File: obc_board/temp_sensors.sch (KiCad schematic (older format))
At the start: 84 parts, among them U10 BMM150, U4 LTC4304CMSTRPBF, U5 MCP9600-E_MX, U6 MCP9600-E_MX, U7 MCP9600-E_MX, U8 MCP9600-E_MX, U9 BMI160

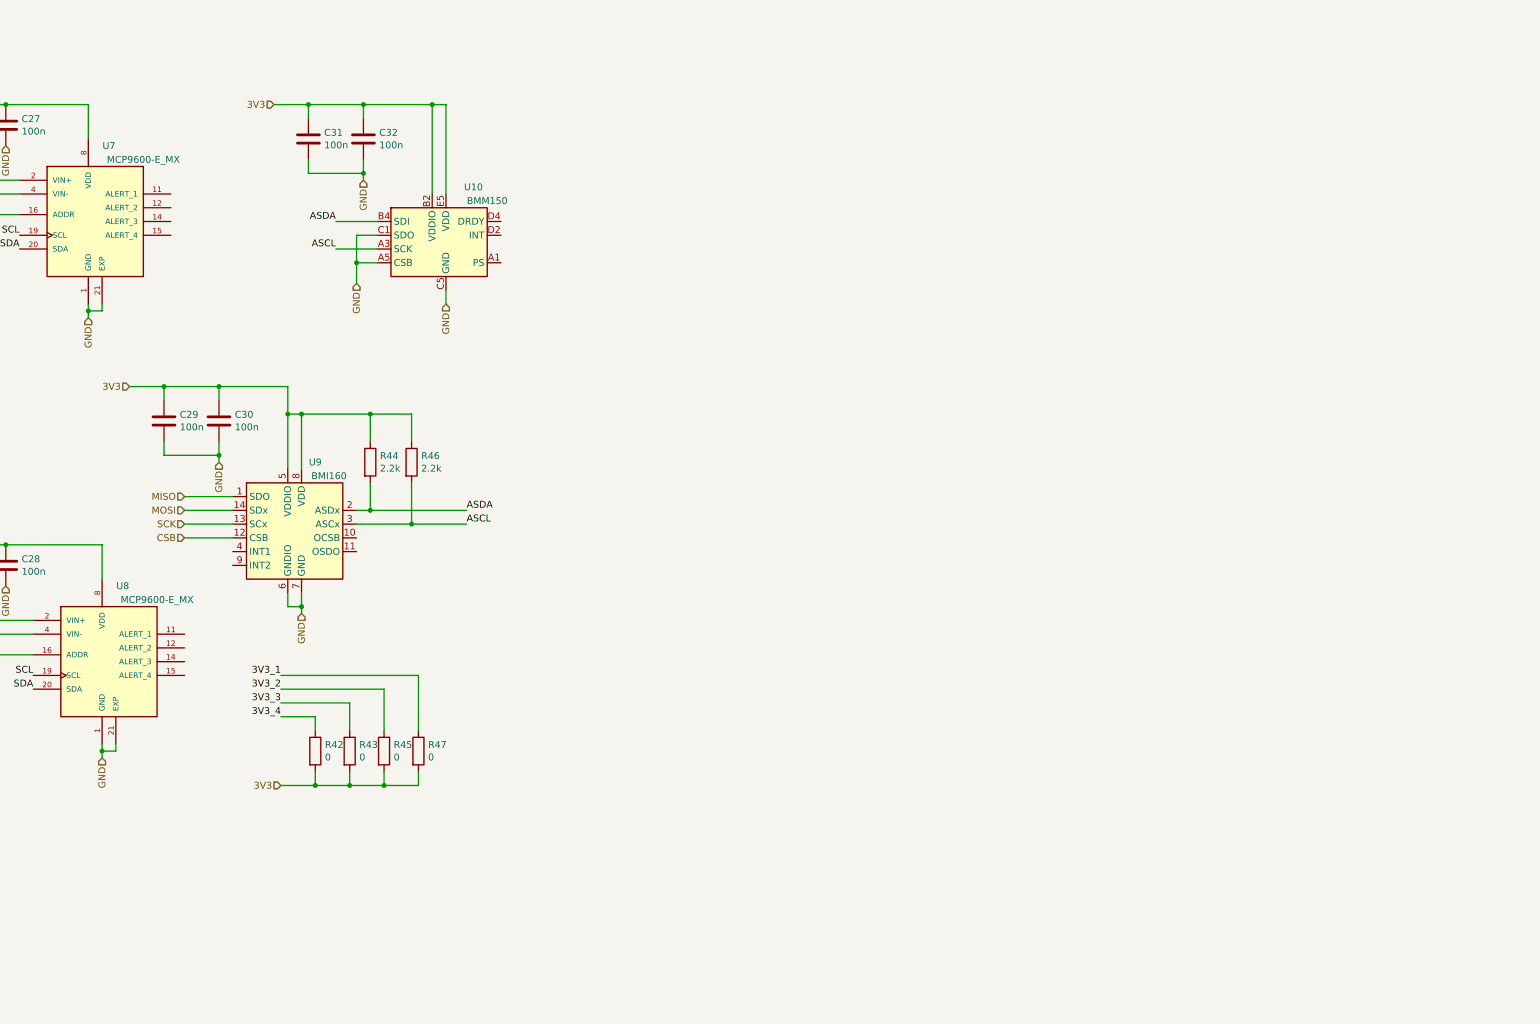
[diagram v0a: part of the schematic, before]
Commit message: modify planes
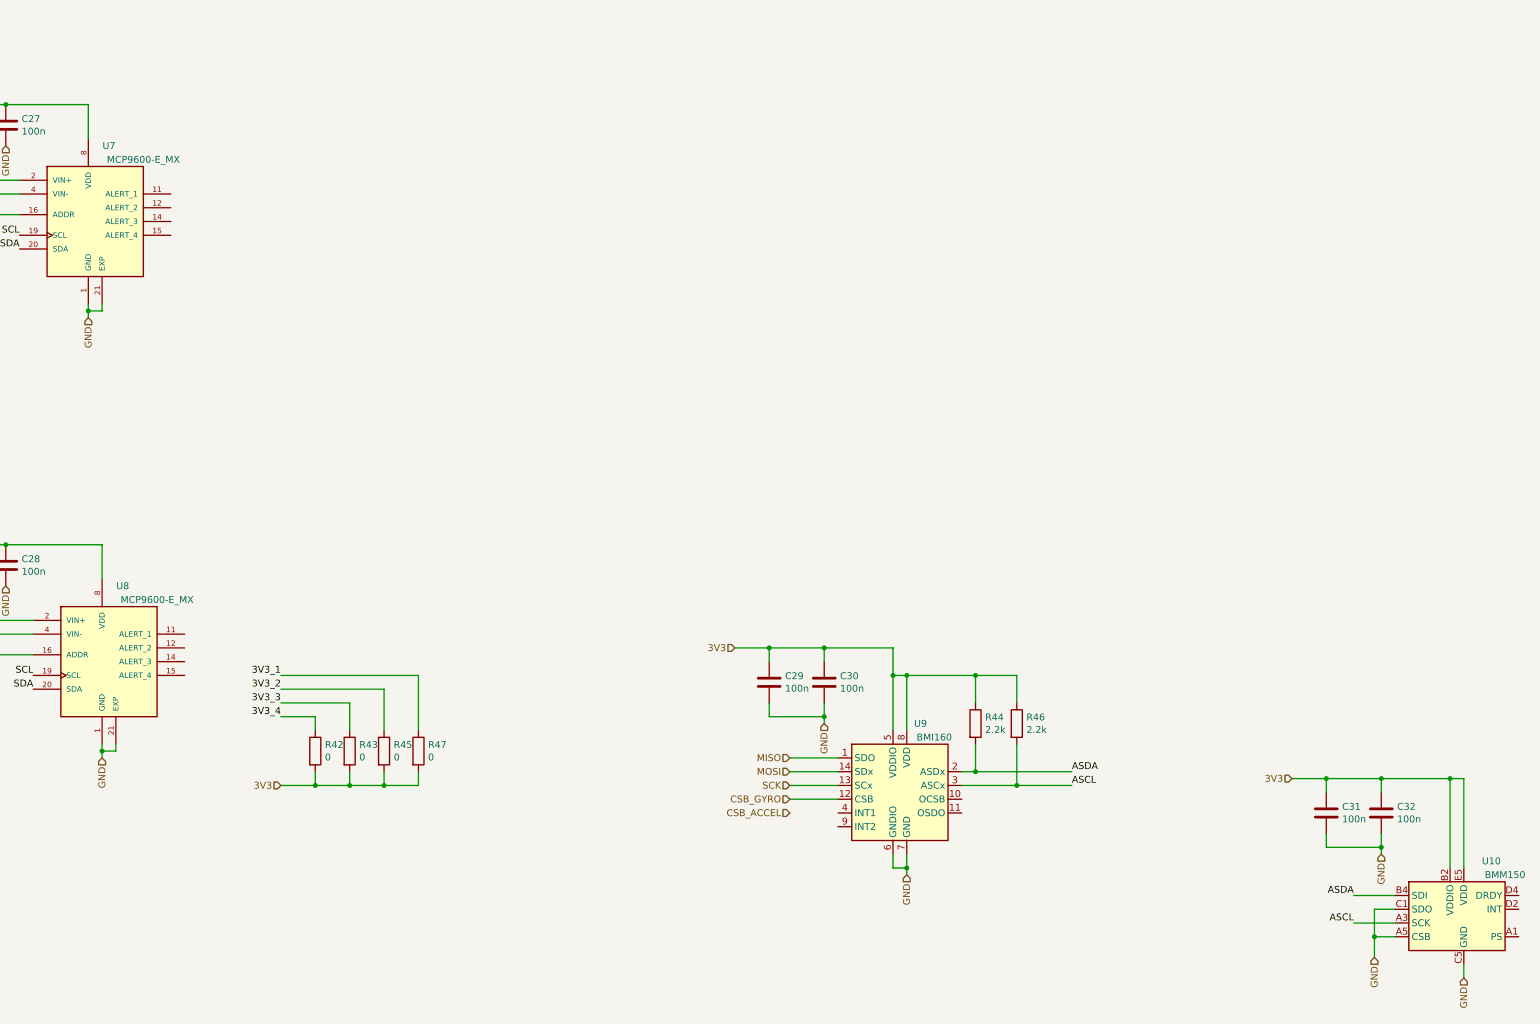
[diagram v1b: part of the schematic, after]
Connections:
- net CSB renamed CSB_GYRO
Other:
- moved on the sheet: C29, C30, C31, C32, R44, R46, U10, U9
